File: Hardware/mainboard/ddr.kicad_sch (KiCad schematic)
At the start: 35 parts, among them U100 MCIMX6Y2DVM09AB, U202 MT41K256M16HA

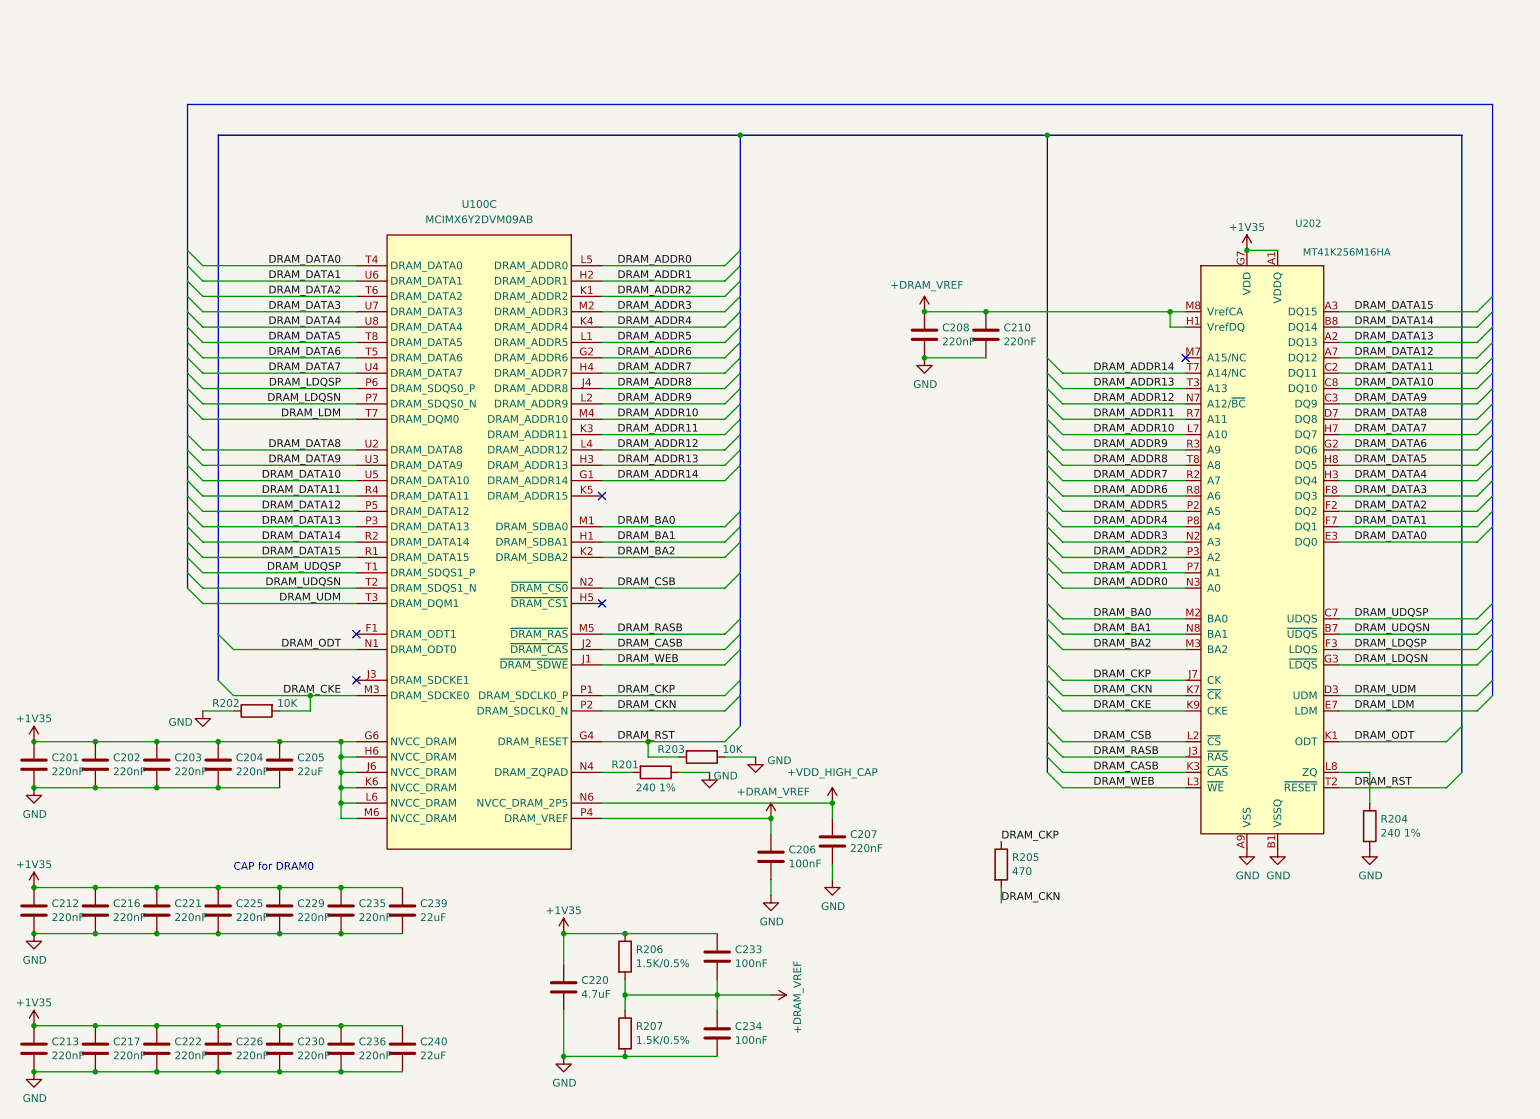
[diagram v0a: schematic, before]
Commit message: New PCB rev
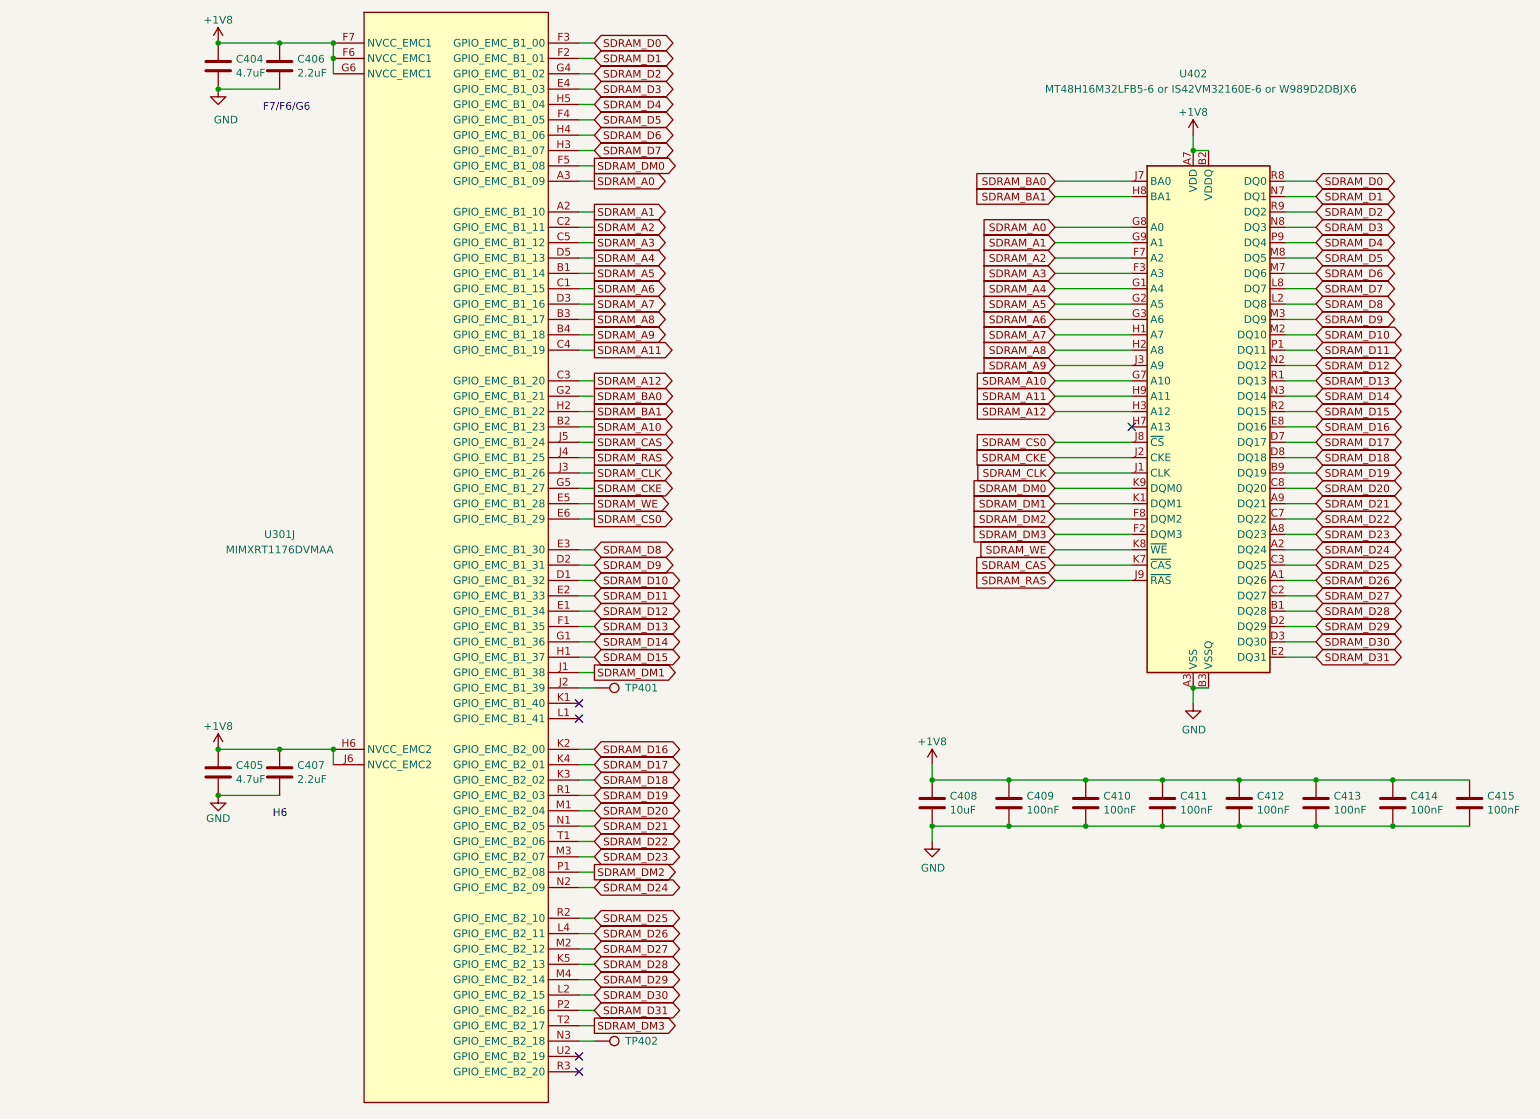
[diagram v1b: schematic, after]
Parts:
- removed C201, C202, C203, C204, C207, C208, C210, C212, C213, C216, C217, C221, C222, C225, C226, C229, C230, C235, C236: 220nF, Capacitor_SMD:C_0402_1005Metric, symbol Device:C
- removed C205, C239, C240: 22uF, Capacitor_SMD:C_0603_1608Metric, symbol Device:C
- removed C206, C233, C234: 100nF, Capacitor_SMD:C_0402_1005Metric, symbol Device:C
- removed C220: 4.7uF, Capacitor_SMD:C_0603_1608Metric, symbol Device:C
- removed R201, R204: 240 1%, Resistor_SMD:R_0402_1005Metric, symbol Device:R
- removed R202, R203: 10K, Resistor_SMD:R_0402_1005Metric, symbol Device:R
- removed R205: 470, Resistor_SMD:R_0402_1005Metric, symbol Device:R
- removed R206, R207: 1.5K/0.5%, Resistor_SMD:R_0402_1005Metric, symbol Device:R
- removed U100: MCIMX6Y2DVM09AB, footprints:BGA-289_17x17_14.0x14.0mm, symbol symbols:MCIMX6Y7DVM09AB
- removed U202: MT41K256M16HA, footprints:BGA-96_9.0x14.0mm_P0.8mm, symbol symbols:MT41K256M16HA
- added C404, C405: 4.7uF, Capacitor_SMD:C_0402_1005Metric, symbol Device:C
- added C406, C407: 2.2uF, Capacitor_SMD:C_0402_1005Metric, symbol Device:C
- added C408: 10uF, Capacitor_SMD:C_0402_1005Metric, symbol Device:C
- added C409, C410, C411, C412, C413, C414, C415: 100nF, Capacitor_SMD:C_0402_1005Metric, symbol Device:C
- added TP401, TP402: TestPoint, footprints:TestPoint_Pad_D0.5mm, symbol Connector:TestPoint
- added U301: MIMXRT1176DVMAA, footprints:BGA-289_17x17_14.0x14.0mm, symbol symbols:MIMXRT1176DVMAA
- added U402: MT48H16M32LFB5-6 or IS42VM32160E-6 or W989D2DBJX6, footprints:BGA-90_9x15_8.0x13.0mm, symbol symbols:IS42S32800J-xB
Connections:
- net GND: now also C404.2, C405.2, C406.2, C407.2, C408.2, C409.2, C410.2, C411.2, C412.2, C413.2, C414.2, C415.2, U402.A3 (VSS), U402.B3 (VSSQ), U402.B8 (VSSQ), U402.C1 (VSSQ), U402.D1 (VSSQ), U402.E9 (VSSQ), U402.F1 (VSS), U402.L3 (VSS), U402.L9 (VSSQ), U402.M1 (VSSQ), U402.N1 (VSSQ), U402.P3 (VSSQ), U402.P8 (VSSQ), U402.R3 (VSS)
- new net: TP401.1, U301.J2 (GPIO_EMC_B1_39)
- new net: TP402.1, U301.N3 (GPIO_EMC_B2_18)
- new net +1V8: C404.1, C405.1, C406.1, C407.1, C408.1, C409.1, C410.1, C411.1, C412.1, C413.1, C414.1, C415.1, U301.F6 (NVCC_EMC1), U301.F7 (NVCC_EMC1), U301.G6 (NVCC_EMC1), U301.H6 (NVCC_EMC2), U301.J6 (NVCC_EMC2), U402.A7 (VDD), U402.B2 (VDDQ), U402.B7 (VDDQ), U402.C9 (VDDQ), U402.D9 (VDDQ), U402.E1 (VDDQ), U402.F9 (VDD), U402.L1 (VDDQ), U402.L7 (VDD), U402.M9 (VDDQ), U402.N9 (VDDQ), U402.P2 (VDDQ), U402.P7 (VDDQ), U402.R7 (VDD)
- new net SDRAM_A0: U301.A3 (GPIO_EMC_B1_09), U402.G8 (A0)
- new net SDRAM_A1: U301.A2 (GPIO_EMC_B1_10), U402.G9 (A1)
- new net SDRAM_A10: U301.B2 (GPIO_EMC_B1_23), U402.G7 (A10)
- new net SDRAM_A11: U301.C4 (GPIO_EMC_B1_19), U402.H9 (A11)
- new net SDRAM_A12: U301.C3 (GPIO_EMC_B1_20), U402.H3 (A12)
- new net SDRAM_A2: U301.C2 (GPIO_EMC_B1_11), U402.F7 (A2)
- new net SDRAM_A3: U301.C5 (GPIO_EMC_B1_12), U402.F3 (A3)
- new net SDRAM_A4: U301.D5 (GPIO_EMC_B1_13), U402.G1 (A4)
- new net SDRAM_A5: U301.B1 (GPIO_EMC_B1_14), U402.G2 (A5)
- new net SDRAM_A6: U301.C1 (GPIO_EMC_B1_15), U402.G3 (A6)
- new net SDRAM_A7: U301.D3 (GPIO_EMC_B1_16), U402.H1 (A7)
- new net SDRAM_A8: U301.B3 (GPIO_EMC_B1_17), U402.H2 (A8)
- new net SDRAM_A9: U301.B4 (GPIO_EMC_B1_18), U402.J3 (A9)
- new net SDRAM_BA0: U301.G2 (GPIO_EMC_B1_21), U402.J7 (BA0)
- new net SDRAM_BA1: U301.H2 (GPIO_EMC_B1_22), U402.H8 (BA1)
- new net SDRAM_CAS: U301.J5 (GPIO_EMC_B1_24), U402.K7 (~{CAS})
- new net SDRAM_CKE: U301.G5 (GPIO_EMC_B1_27), U402.J2 (CKE)
- new net SDRAM_CLK: U301.J3 (GPIO_EMC_B1_26), U402.J1 (CLK)
- new net SDRAM_CS0: U301.E6 (GPIO_EMC_B1_29), U402.J8 (~{CS})
- new net SDRAM_D0: U301.F3 (GPIO_EMC_B1_00), U402.R8 (DQ0)
- new net SDRAM_D1: U301.F2 (GPIO_EMC_B1_01), U402.N7 (DQ1)
- new net SDRAM_D10: U301.D1 (GPIO_EMC_B1_32), U402.M2 (DQ10)
- new net SDRAM_D11: U301.E2 (GPIO_EMC_B1_33), U402.P1 (DQ11)
- new net SDRAM_D12: U301.E1 (GPIO_EMC_B1_34), U402.N2 (DQ12)
- new net SDRAM_D13: U301.F1 (GPIO_EMC_B1_35), U402.R1 (DQ13)
- new net SDRAM_D14: U301.G1 (GPIO_EMC_B1_36), U402.N3 (DQ14)
- new net SDRAM_D15: U301.H1 (GPIO_EMC_B1_37), U402.R2 (DQ15)
- new net SDRAM_D16: U301.K2 (GPIO_EMC_B2_00), U402.E8 (DQ16)
- new net SDRAM_D17: U301.K4 (GPIO_EMC_B2_01), U402.D7 (DQ17)
- new net SDRAM_D18: U301.K3 (GPIO_EMC_B2_02), U402.D8 (DQ18)
- new net SDRAM_D19: U301.R1 (GPIO_EMC_B2_03), U402.B9 (DQ19)
- new net SDRAM_D2: U301.G4 (GPIO_EMC_B1_02), U402.R9 (DQ2)
- new net SDRAM_D20: U301.M1 (GPIO_EMC_B2_04), U402.C8 (DQ20)
- new net SDRAM_D21: U301.N1 (GPIO_EMC_B2_05), U402.A9 (DQ21)
- new net SDRAM_D22: U301.T1 (GPIO_EMC_B2_06), U402.C7 (DQ22)
- new net SDRAM_D23: U301.M3 (GPIO_EMC_B2_07), U402.A8 (DQ23)
- new net SDRAM_D24: U301.N2 (GPIO_EMC_B2_09), U402.A2 (DQ24)
- new net SDRAM_D25: U301.R2 (GPIO_EMC_B2_10), U402.C3 (DQ25)
- new net SDRAM_D26: U301.L4 (GPIO_EMC_B2_11), U402.A1 (DQ26)
- new net SDRAM_D27: U301.M2 (GPIO_EMC_B2_12), U402.C2 (DQ27)
- new net SDRAM_D28: U301.K5 (GPIO_EMC_B2_13), U402.B1 (DQ28)
- new net SDRAM_D29: U301.M4 (GPIO_EMC_B2_14), U402.D2 (DQ29)
- new net SDRAM_D3: U301.E4 (GPIO_EMC_B1_03), U402.N8 (DQ3)
- new net SDRAM_D30: U301.L2 (GPIO_EMC_B2_15), U402.D3 (DQ30)
- new net SDRAM_D31: U301.P2 (GPIO_EMC_B2_16), U402.E2 (DQ31)
- new net SDRAM_D4: U301.H5 (GPIO_EMC_B1_04), U402.P9 (DQ4)
- new net SDRAM_D5: U301.F4 (GPIO_EMC_B1_05), U402.M8 (DQ5)
- new net SDRAM_D6: U301.H4 (GPIO_EMC_B1_06), U402.M7 (DQ6)
- new net SDRAM_D7: U301.H3 (GPIO_EMC_B1_07), U402.L8 (DQ7)
- new net SDRAM_D8: U301.E3 (GPIO_EMC_B1_30), U402.L2 (DQ8)
- new net SDRAM_D9: U301.D2 (GPIO_EMC_B1_31), U402.M3 (DQ9)
- new net SDRAM_DM0: U301.F5 (GPIO_EMC_B1_08), U402.K9 (DQM0)
- new net SDRAM_DM1: U301.J1 (GPIO_EMC_B1_38), U402.K1 (DQM1)
- new net SDRAM_DM2: U301.P1 (GPIO_EMC_B2_08), U402.F8 (DQM2)
- new net SDRAM_DM3: U301.T2 (GPIO_EMC_B2_17), U402.F2 (DQM3)
- new net SDRAM_RAS: U301.J4 (GPIO_EMC_B1_25), U402.J9 (~{RAS})
- new net SDRAM_WE: U301.E5 (GPIO_EMC_B1_28), U402.K8 (~{WE})
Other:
- note added: "F7/F6/G6"
- note added: "H6"
- note removed: "CAP for DRAM0"
